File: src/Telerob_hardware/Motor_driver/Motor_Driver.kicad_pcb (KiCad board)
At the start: 2 copper layers, 22 parts

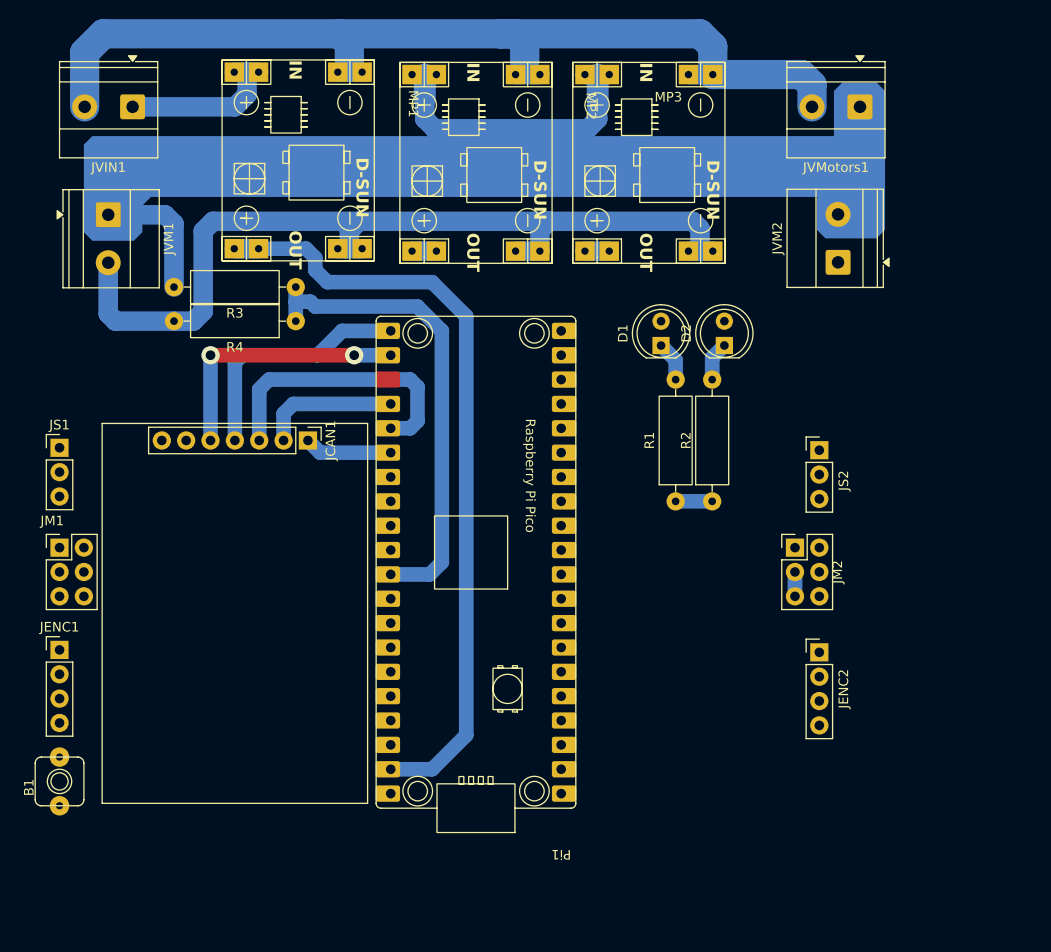
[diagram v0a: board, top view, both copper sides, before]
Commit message: Codes
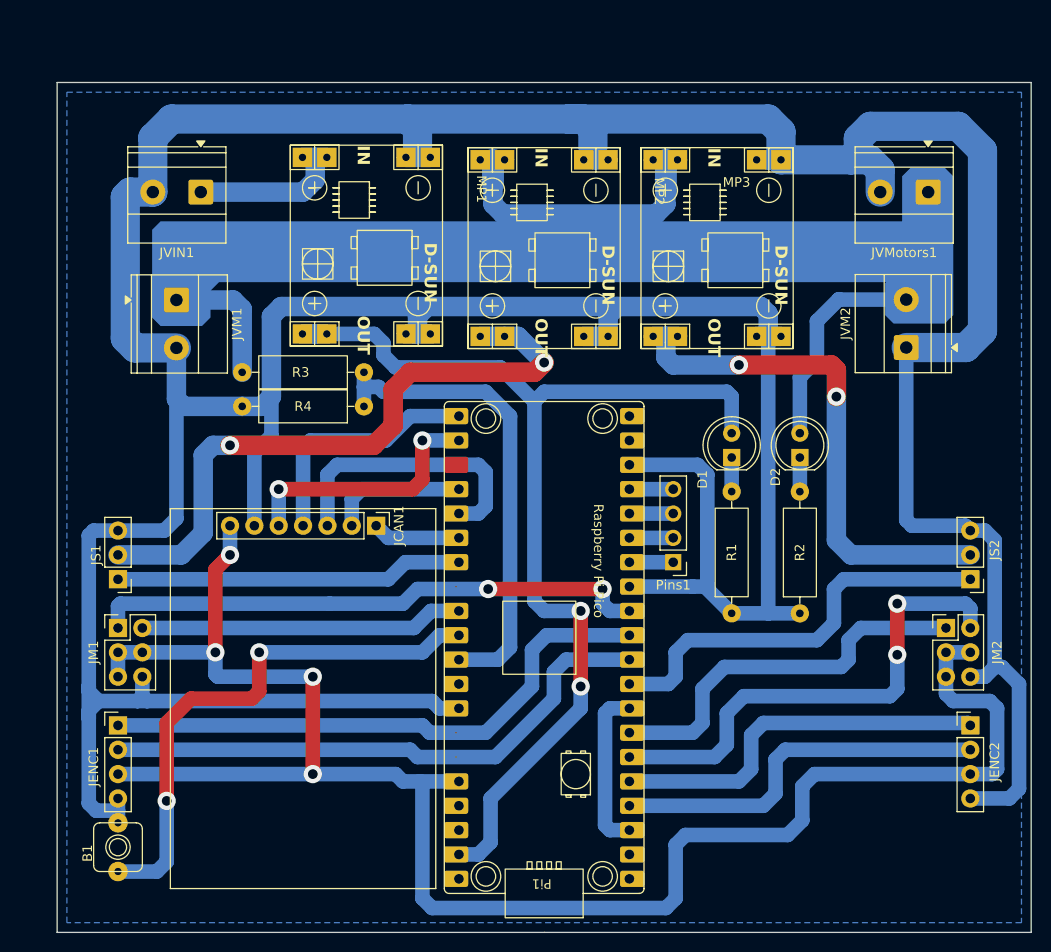
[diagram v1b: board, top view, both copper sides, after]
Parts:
- added Pins1: ~, Connector_PinHeader_2.54mm:PinHeader_1x04_P2.54mm_Vertical, F.Cu at (162.8, 99.8)
- moved JS2 20.7 mm to (193.8, 101.6), turned to 180 degrees
- moved JM2 17.8 mm to (191.3, 106.7)
- moved JENC2 17.5 mm to (193.8, 116.8)
- moved JS1 15.0 mm to (104.9, 101.6), turned to 180 degrees
- moved R2 14.8 mm to (176.0, 105.2)
- moved D2 14.1 mm to (176.0, 88.9)
- moved D1 13.8 mm to (168.9, 88.9)
- moved R1 13.1 mm to (168.9, 105.2)
- moved MP3 11.4 mm to (174.1, 57.8)
- moved JVM1 11.4 mm to (111.0, 72.5)
- moved R3 11.4 mm to (130.6, 80.0)
- moved R4 11.4 mm to (130.6, 83.6)
- moved JCAN1 11.4 mm to (131.8, 96.0)
- moved JVIN1 11.4 mm to (113.5, 61.2)
- moved JVM2 11.4 mm to (187.1, 77.4)
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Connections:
- JM1 pad 1: /GP4 -> /GP9
- JM1 pad 2: /3V3_O -> /GP22
- JM1 pad 4: /GP5 -> /3V3_O
- JM2 pad 1: /GP2 -> /GP5
- JM2 pad 2: /3V3_O -> /GP4
- JM2 pad 4: /GP3 -> /3V3_O
- JS1 pad 1: /GP5 -> /GP21
- Pi1 pad 10: /GP8 -> /B_1
- Pi1 pad 3: /GP2 -> /A_2
- Pi1 pad 4: /GP3 -> /B_2
- Pi1 pad 9: /GP7 -> /A_1
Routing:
- net /GND: track 202.5 -> 532.0 mm
- net /3V3_O: track 2.54 -> 188.3 mm, vias 0 -> 4
- net /5V_S1: track 2.54 -> 67.6 mm, vias 0 -> 2
- net /B_1: track 0.00 -> 60.1 mm
- net /A_1: track 0.00 -> 59.5 mm
- net /GP9: track 0.00 -> 58.2 mm, vias 0 -> 2
- net /RUN: track 0.00 -> 56.6 mm, vias 0 -> 2
- net /5V_S2: track 2.54 -> 55.4 mm, vias 0 -> 2
- net /GP4: track 0.00 -> 51.7 mm, vias 0 -> 2
- net /GP6: track 0.00 -> 43.7 mm
- net /GP5: track 0.00 -> 40.8 mm
- net /B_2: track 0.00 -> 40.3 mm
- net /A_2: track 0.00 -> 40.1 mm
- net /GP21: track 0.00 -> 36.3 mm
- net /GP22: track 0.00 -> 33.8 mm
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- added copper zone on B.Cu, net /GND
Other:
- board outline added: 101.6 x 88.6 mm
